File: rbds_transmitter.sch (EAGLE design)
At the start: 98 parts, among them IC1 MAX1551, IC2 TPS61030, IC3 MCP4812, IC4 OPA4743UA, IC5 OPA4743UA, Q1 P-Ch, Q2 P-CH, SW1 FSMSM, U3 ATMEGA328, X1 HD44780LCD-1602, Y1 16Mhz

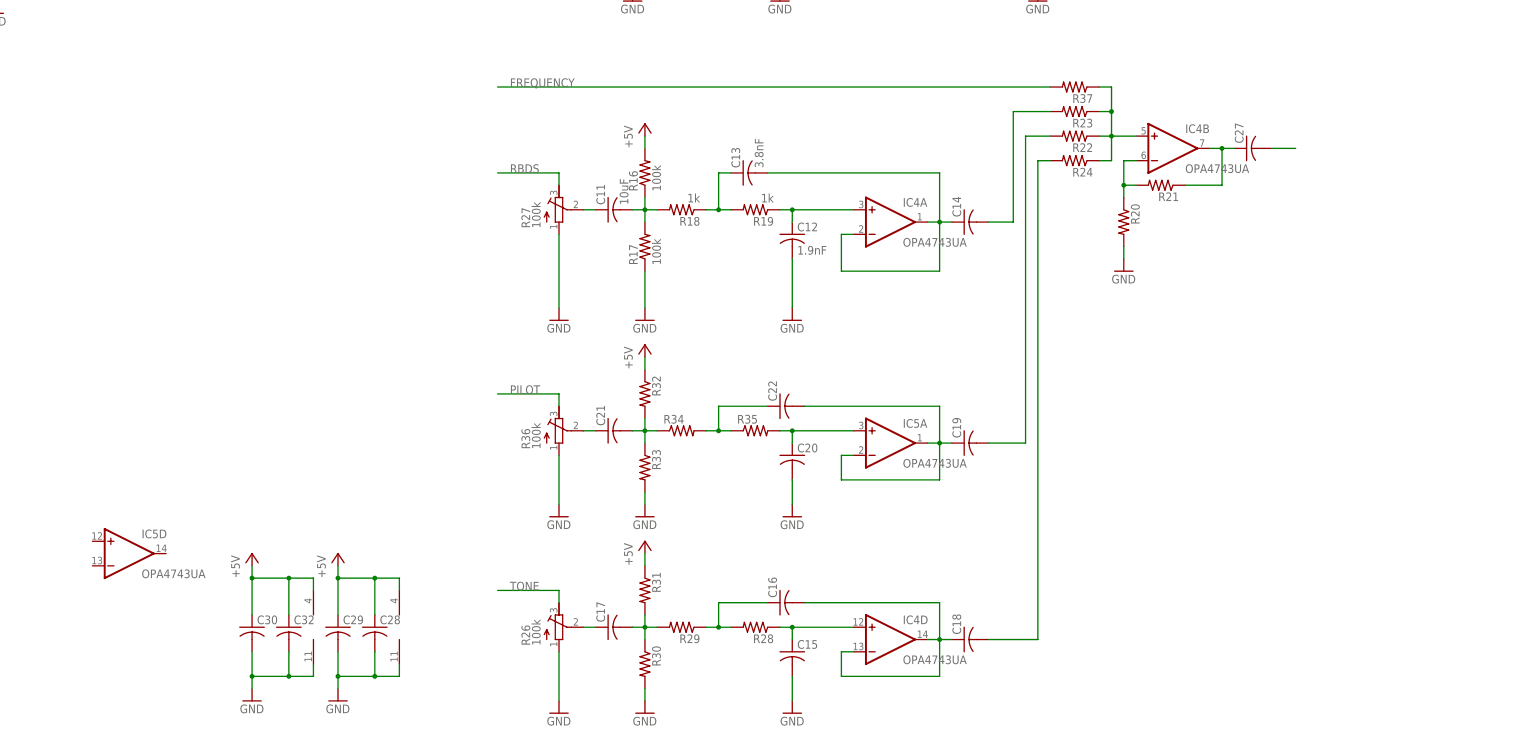
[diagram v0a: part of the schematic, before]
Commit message: still working
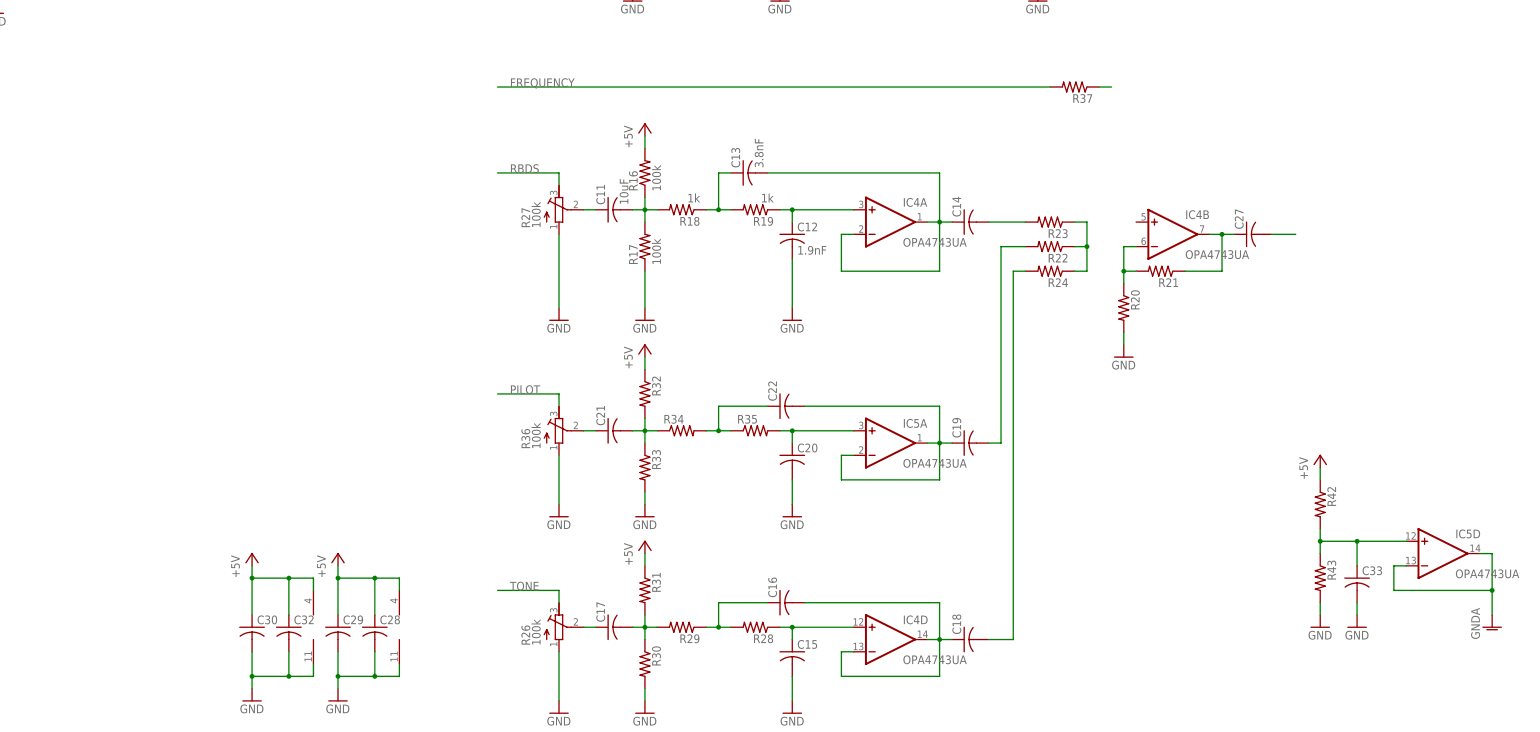
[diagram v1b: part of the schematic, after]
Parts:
- added C33: (no value), adafruit:C-USC1206
- added R42, R43: (no value), adafruit:R-US_R1206
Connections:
- new net GNDA: IC5D.-IN, IC5D.OUT
- new net N$29: C33.1, IC5D.+IN, R42.2, R43.1
- new net N$5: R37.1
- net +5V: now also R42.1
- net GND: now also C33.2, R43.2
- net N$27: no longer IC4B.+IN, R37.1
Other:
- moved on the sheet: C27, IC4B, IC5D, R20, R21, R22, R23, R24
